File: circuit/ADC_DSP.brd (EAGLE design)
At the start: 40.3 x 57.8 mm, 51 parts, among them IC1 REG1117, IC3 STM32F40XRXT6, IC4 CS4272, Q1 8MHz, Q2 24.576MHz

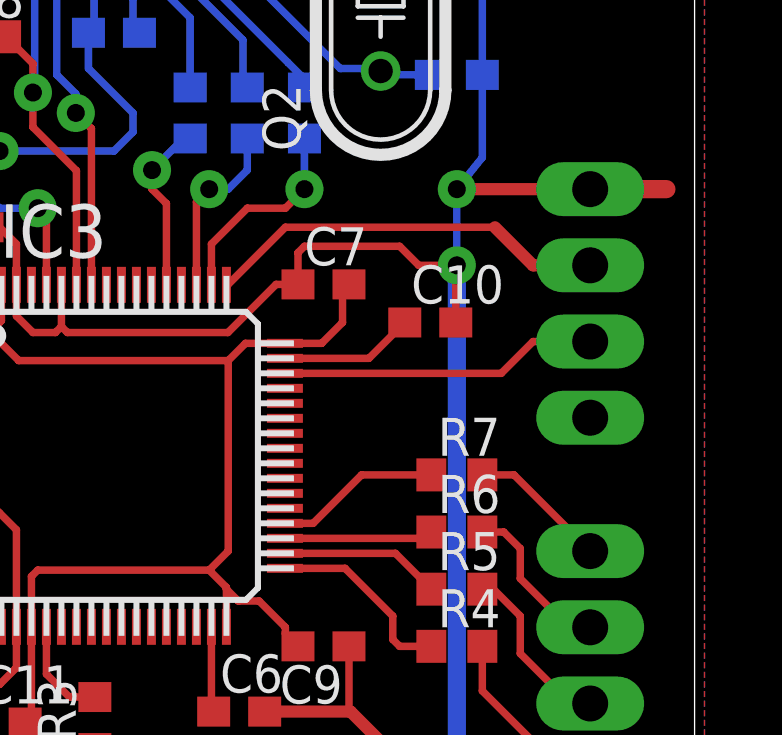
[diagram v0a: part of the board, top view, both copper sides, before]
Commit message: - ?????? ?????????? ? ?????????????? ??????????????????
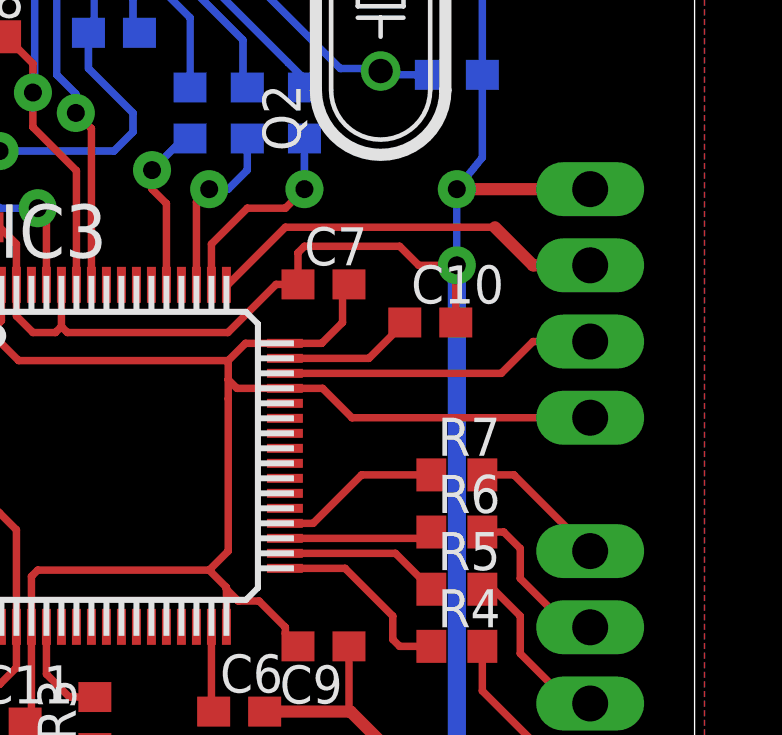
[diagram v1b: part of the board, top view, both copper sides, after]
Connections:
- net +3V3: now also IC3.45
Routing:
- net +3V3: track 96.3 -> 108.9 mm
- net GND: track 163.3 -> 160.8 mm
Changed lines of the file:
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@@
 <setting verticaltext="up"/>
 </settings>
-<grid distance="0.635" unitdist="mm" unit="mm" style="lines" multiple="1" display="no" altdistance="0.25" altunitdist="mm" altunit="mm"/>
+<grid distance="0.635" unitdist="mm" unit="mm" style="lines" multiple="1" display="no" altdistance="0.125" altunitdist="mm" altunit="mm"/>
 <layers>
 <layer number="1" name="Top" color="4" fill="1" visible="yes" active="yes"/>
@@
 <wire x1="8.89" y1="16.19" x2="8.89" y2="16.51" width="0.4064" layer="1"/>
 <wire x1="8.89" y1="16.51" x2="7.7775" y2="17.6225" width="0.4064" layer="1"/>
-<wire x1="39.37" y1="30.48" x2="36.83" y2="30.48" width="0.6096" layer="1"/>
 <wire x1="29.845" y1="7.62" x2="27.305" y2="7.62" width="0.6096" layer="1"/>
 <wire x1="29.845" y1="7.62" x2="32.385" y2="7.62" width="0.6096" layer="1"/>
@@
 <wire x1="26.655" y1="25.34" x2="25.34" y2="25.34" width="0.25" layer="1"/>
 <wire x1="25.34" y1="25.34" x2="24.765" y2="24.765" width="0.25" layer="1"/>
-<wire x1="24.765" y1="24.765" x2="24.765" y2="18.415" width="0.25" layer="1"/>
+<wire x1="24.765" y1="24.765" x2="24.765" y2="24.13" width="0.25" layer="1"/>
+<wire x1="24.765" y1="24.13" x2="24.765" y2="23.495" width="0.25" layer="1"/>
+<wire x1="24.765" y1="23.495" x2="24.765" y2="18.415" width="0.25" layer="1"/>
 <wire x1="24.765" y1="18.415" x2="24.13" y2="17.78" width="0.25" layer="1"/>
 <wire x1="17.205" y1="27.29" x2="15.89" y2="27.29" width="0.25" layer="1"/>
@@
 <wire x1="26.67" y1="15.875" x2="26.67" y2="15.66" width="0.25" layer="1"/>
 <wire x1="26.67" y1="15.66" x2="27.09" y2="15.24" width="0.25" layer="1"/>
-<wire x1="28.575" y1="26.035" x2="36.83" y2="22.86" width="0" layer="19" extent="1-1"/>
+<wire x1="36.83" y1="22.86" x2="28.89" y2="22.86" width="0.25" layer="1"/>
+<contactref element="IC3" pad="45"/>
+<wire x1="26.655" y1="23.84" x2="25.055" y2="23.84" width="0.25" layer="1"/>
+<wire x1="25.055" y1="23.84" x2="24.765" y2="24.13" width="0.25" layer="1"/>
+<wire x1="26.655" y1="23.84" x2="27.91" y2="23.84" width="0.25" layer="1"/>
+<wire x1="27.91" y1="23.84" x2="28.89" y2="22.86" width="0.25" layer="1"/>
 </signal>
 <signal name="N$1">
